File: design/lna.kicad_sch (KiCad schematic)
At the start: 19 parts, among them J5 SMA, U10 ADA4930-1

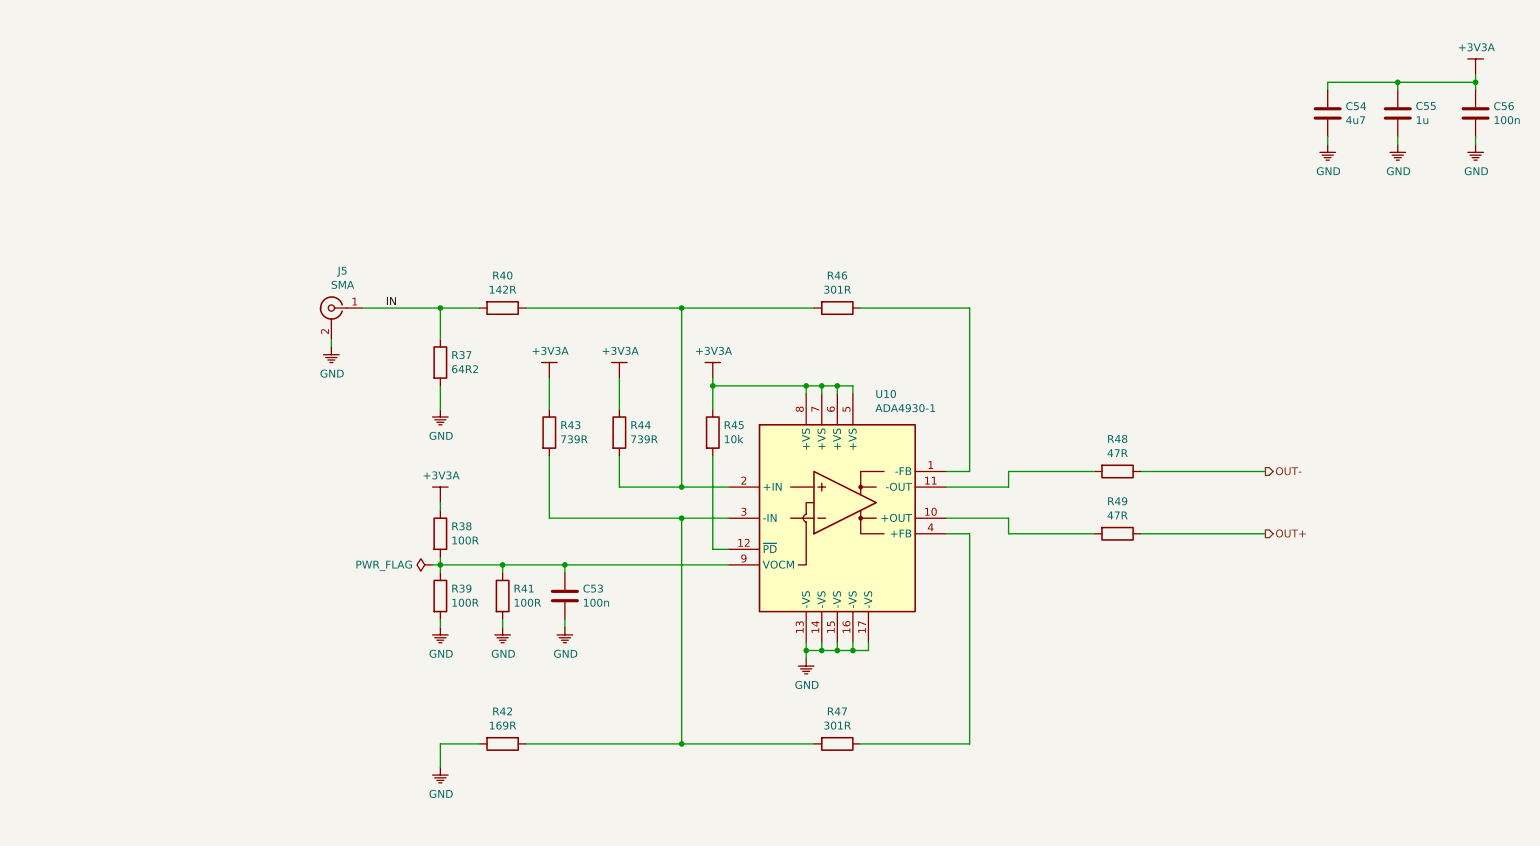
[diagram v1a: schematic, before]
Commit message: Updated schematic
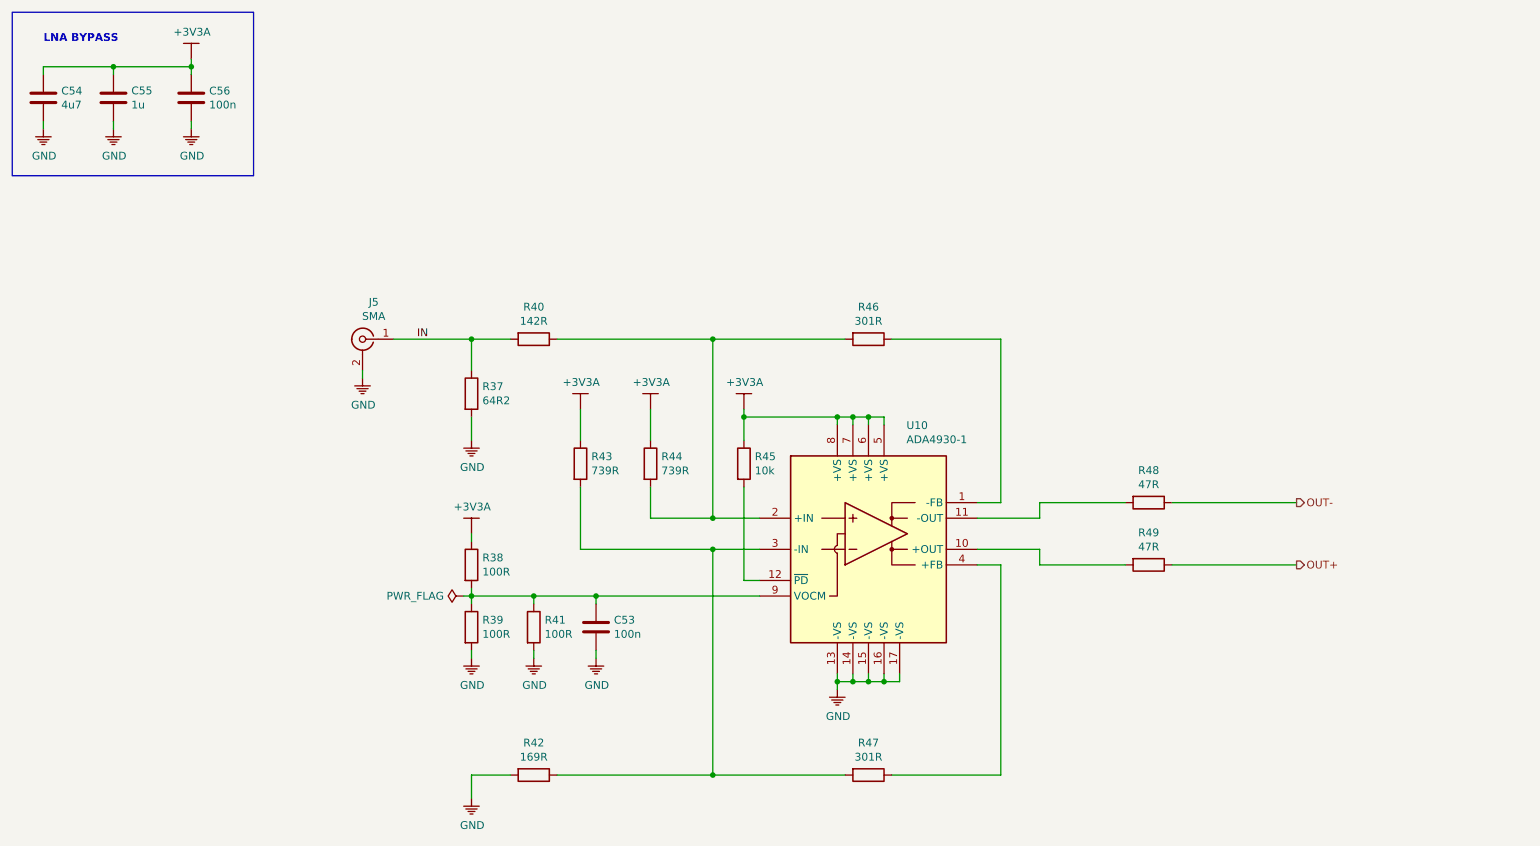
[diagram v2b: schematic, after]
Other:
- note added: "LNA BYPASS"
- moved on the sheet: C53, C54, C55, C56, J5, R37, R38, R39, R40, R41, R42, R43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
